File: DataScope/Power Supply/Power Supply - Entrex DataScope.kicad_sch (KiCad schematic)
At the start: 128 parts, among them J2 Power Port, Q1 MPS3638, Q10 PN3569, Q11 PS3638, Q12 2N4918, Q13 2N3055, Q14 PN3569, Q15 PS3638, Q16 PN3569, Q17 PN3569, Q18 PS3638, Q19 JE520, Q2 PN3569, Q20 PN3569, Q3 PN3569, Q4 PS3638, Q5 2N4918, Q6 2N3055, Q7 PN3569, Q8 PS3638, Q9 PN3569

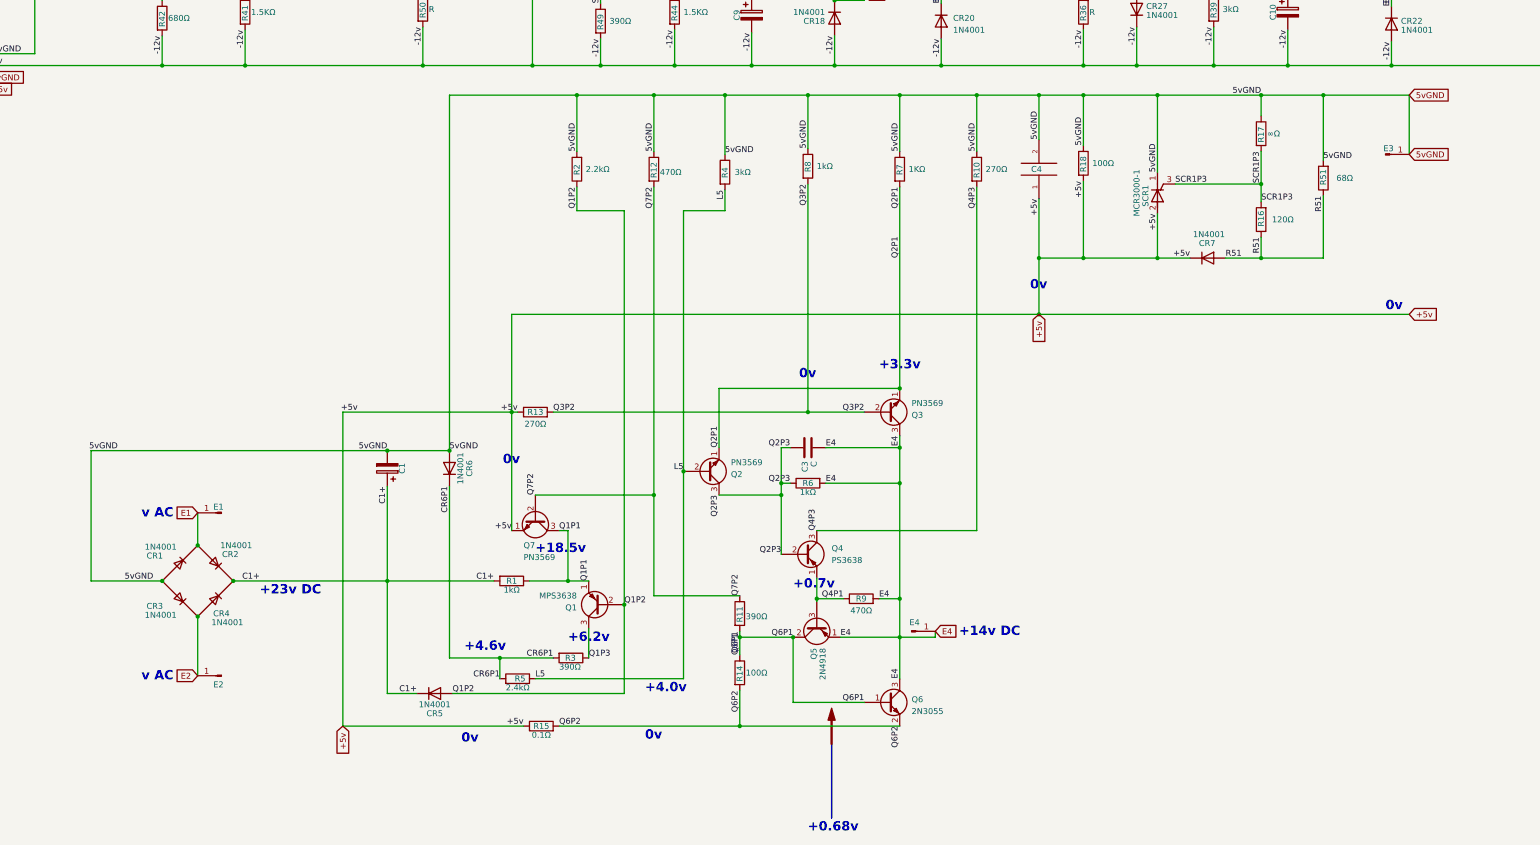
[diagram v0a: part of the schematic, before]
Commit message: diagnose
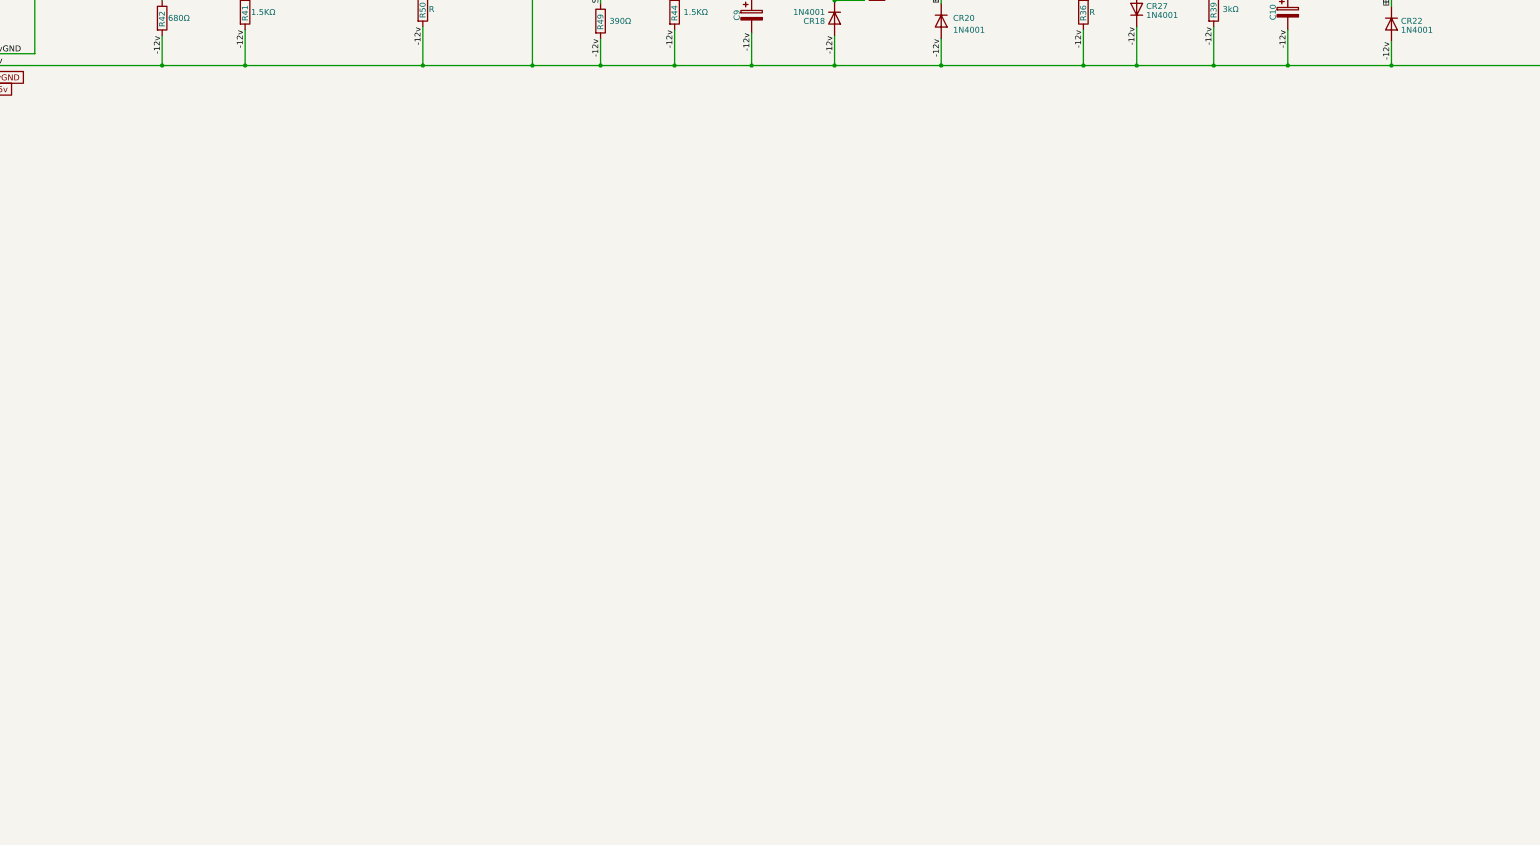
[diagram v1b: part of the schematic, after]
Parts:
- removed C1: C_Polarized, Capacitor_THT:CP_Radial_D10.0mm_P5.00mm, symbol Device:C_Polarized
- removed C3: C, FM-editable:CAP non-polarized P25.00mm, symbol Device:C
- removed C4: CAP, Capacitor_THT:CP_Axial_L20.0mm_D10.0mm_P26.00mm_Horizontal, symbol Forgotten Machines:CAP_Large_Polarized_-_Entrex_Trapezoid
- removed CR1, CR2, CR3, CR4: 1N4001, Diode_THT:D_DO-41_SOD81_P12.70mm_Horizontal, symbol ForgottenMachines:Diagonal Diode for Full Wave Bridge Lower
- removed CR5, CR6, CR7: 1N4001, Diode_THT:D_DO-41_SOD81_P12.70mm_Horizontal, symbol ForgottenMachines:1N4001_Entrex_PSU
- removed E1, E2, E3, E4: Conn_01x01_Pin, Connector_PinHeader_1.00mm:PinHeader_1x01_P1.00mm_Vertical, symbol ForgottenMachines:Spade_Lug_Connector_-_Entrex_PSU
- removed Q1: MPS3638, Package_TO_SOT_THT:TO-18-3, symbol ForgottenMachines:MPS3638_Transistor
- removed Q2, Q3, Q7: PN3569, Package_TO_SOT_THT:TO-18-3, symbol ForgottenMachines:FPN3569_Transistor
- removed Q4: PS3638, Package_TO_SOT_THT:TO-18-3, symbol ForgottenMachines:MPS3638_Transistor
- removed Q5: 2N4918, Package_TO_SOT_THT:TO-126-3_Vertical, symbol Forgotten Machines:2N4918
- removed Q6: 2N3055, Package_TO_SOT_THT:TO-3, symbol Transistor_BJT:2N3055
- removed R1, R6: 1kΩ, Resistor_THT:R_Axial_DIN0309_L9.0mm_D3.2mm_P12.70mm_Horizontal, symbol Device:R
- removed R10, R13: 270Ω, Resistor_THT:R_Axial_DIN0411_L9.9mm_D3.6mm_P12.70mm_Horizontal, symbol Device:R
- removed R11: 390Ω, Resistor_THT:R_Axial_DIN0411_L9.9mm_D3.6mm_P15.24mm_Horizontal, symbol Device:R
- removed R12, R9: 470Ω, Resistor_THT:R_Axial_DIN0309_L9.0mm_D3.2mm_P12.70mm_Horizontal, symbol Device:R
- removed R14: 100Ω, Resistor_THT:R_Axial_DIN0309_L9.0mm_D3.2mm_P12.70mm_Horizontal, symbol Device:R
- removed R15: 0.1Ω, Resistor_THT:R_Axial_DIN0614_L14.3mm_D5.7mm_P20.32mm_Horizontal, symbol Device:R
- removed R16: 120Ω, Resistor_THT:R_Axial_DIN0614_L14.3mm_D5.7mm_P15.24mm_Horizontal, symbol Device:R
- removed R17: ∞Ω, Resistor_THT:R_Axial_DIN0309_L9.0mm_D3.2mm_P12.70mm_Horizontal, symbol Device:R
- removed R18: 100Ω, Resistor_THT:R_Axial_DIN0614_L14.3mm_D5.7mm_P15.24mm_Horizontal, symbol Device:R
- removed R2: 2.2kΩ, Resistor_THT:R_Axial_DIN0411_L9.9mm_D3.6mm_P12.70mm_Horizontal, symbol Device:R
- removed R3: 390Ω, Resistor_THT:R_Axial_DIN0411_L9.9mm_D3.6mm_P12.70mm_Horizontal, symbol Device:R
- removed R4: 3kΩ, Resistor_THT:R_Axial_DIN0309_L9.0mm_D3.2mm_P12.70mm_Horizontal, symbol Device:R
- removed R5: 2.4kΩ, Resistor_THT:R_Axial_DIN0309_L9.0mm_D3.2mm_P12.70mm_Horizontal, symbol Device:R
- removed R51: 68Ω, Resistor_THT:R_Axial_DIN0411_L9.9mm_D3.6mm_P12.70mm_Horizontal, symbol Device:R
- removed R7: 1KΩ, Resistor_THT:R_Axial_DIN0411_L9.9mm_D3.6mm_P12.70mm_Horizontal, symbol Device:R
- removed R8: 1kΩ, Resistor_THT:R_Axial_DIN0411_L9.9mm_D3.6mm_P12.70mm_Horizontal, symbol Device:R
- removed SCR1: MCR3000-1, Package_TO_SOT_THT:TO-126-3_Vertical, symbol ForgottenMachines:MCR3000-1
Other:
- note removed: "+0.68v"
- note removed: "+0.7v"
- note removed: "+14v DC"
- note removed: "+18.5v"
- note removed: "+23v DC"
- note removed: "+3.3v"
- note removed: "+4.0v"
- note removed: "+4.6v"
- note removed: "+6.2v"
- note removed: "0v"
- note removed: "v AC"
